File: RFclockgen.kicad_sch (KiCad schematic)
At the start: 1 part, among them U1 ADF4351BCPZ-RL7

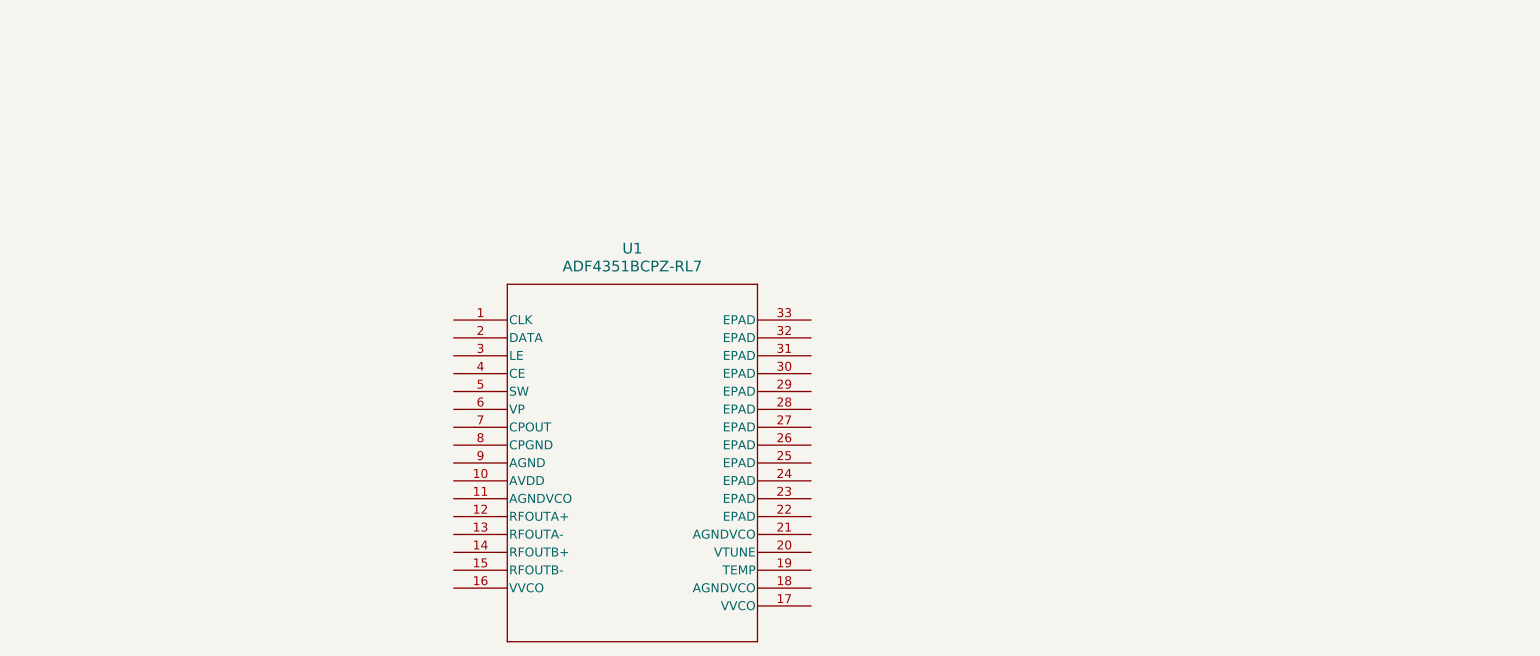
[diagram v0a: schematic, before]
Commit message: Added more components!
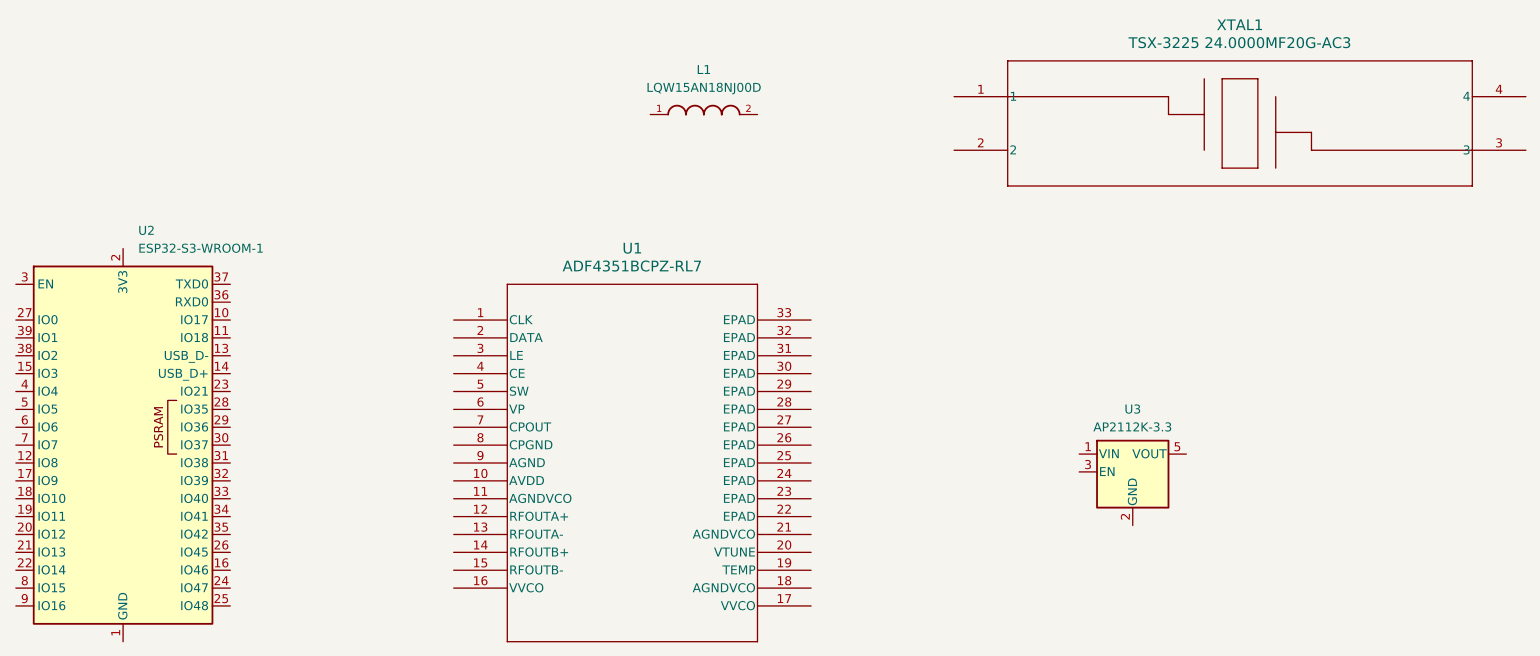
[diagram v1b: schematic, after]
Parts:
- added L1: LQW15AN18NJ00D, LQW15AN18NJ00D:INDC1006X60N, symbol LQW15AN18NJ00D:LQW15AN18NJ00D
- added U2: ESP32-S3-WROOM-1, RF_Module:ESP32-S3-WROOM-1, symbol RF_Module:ESP32-S3-WROOM-1
- added U3: AP2112K-3.3, Package_TO_SOT_SMD:SOT-23-5, symbol Regulator_Linear:AP2112K-3.3
- added XTAL1: TSX-3225 24.0000MF20G-AC3, TSX-3225 24.0000MF20G-AC3_EPS, symbol TSX_3225_24_0000MF20G_AC3:TSX-3225_24.0000MF20G-AC3
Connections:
- new net: U2.1 (GND), U2.40 (GND), U2.41 (GND)
